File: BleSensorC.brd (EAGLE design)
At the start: 29 x 40.5 mm, 20 parts, among them IC1 PIC16LF18446-I_SS, IC2 SI7020-A20-GM, Q1 SI2333DDS-T1-GE3, T1 VEMT2523SLX01, U1 RN4871-I

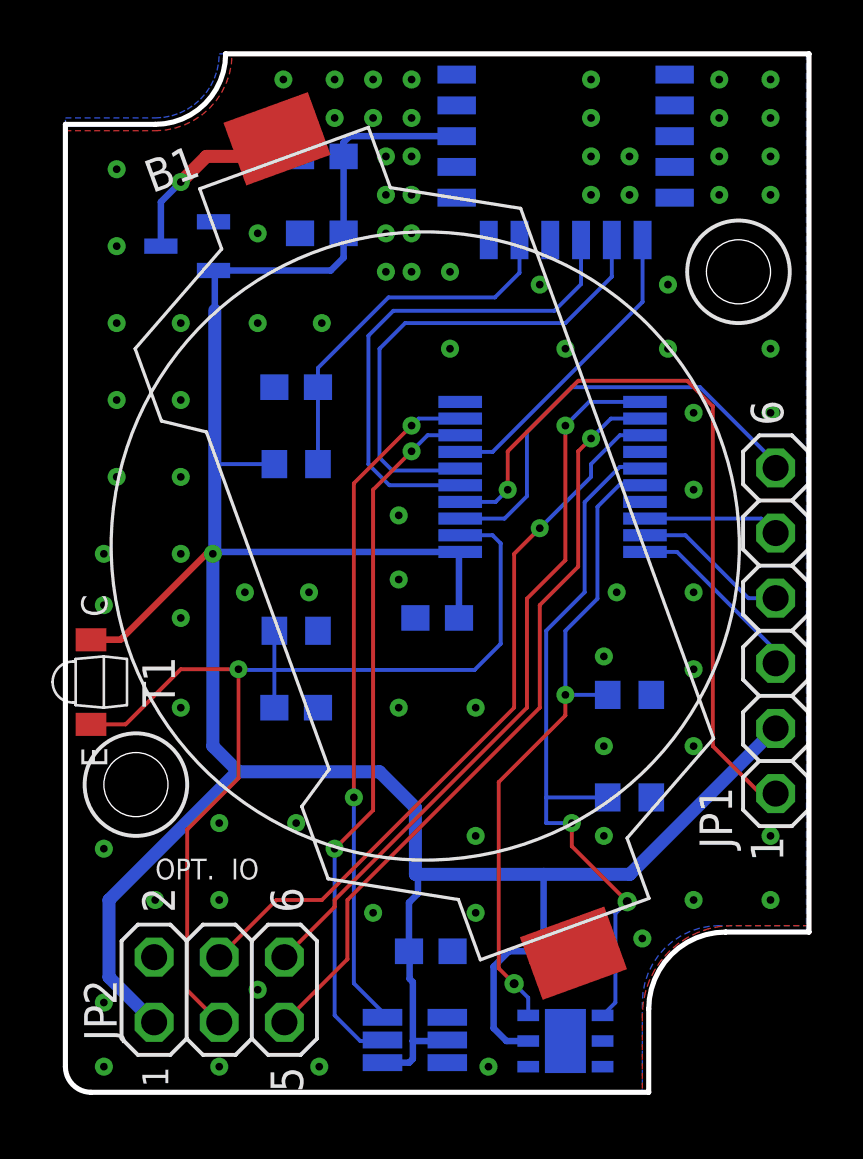
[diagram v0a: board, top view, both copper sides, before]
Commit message: U1 placing
U1 placing
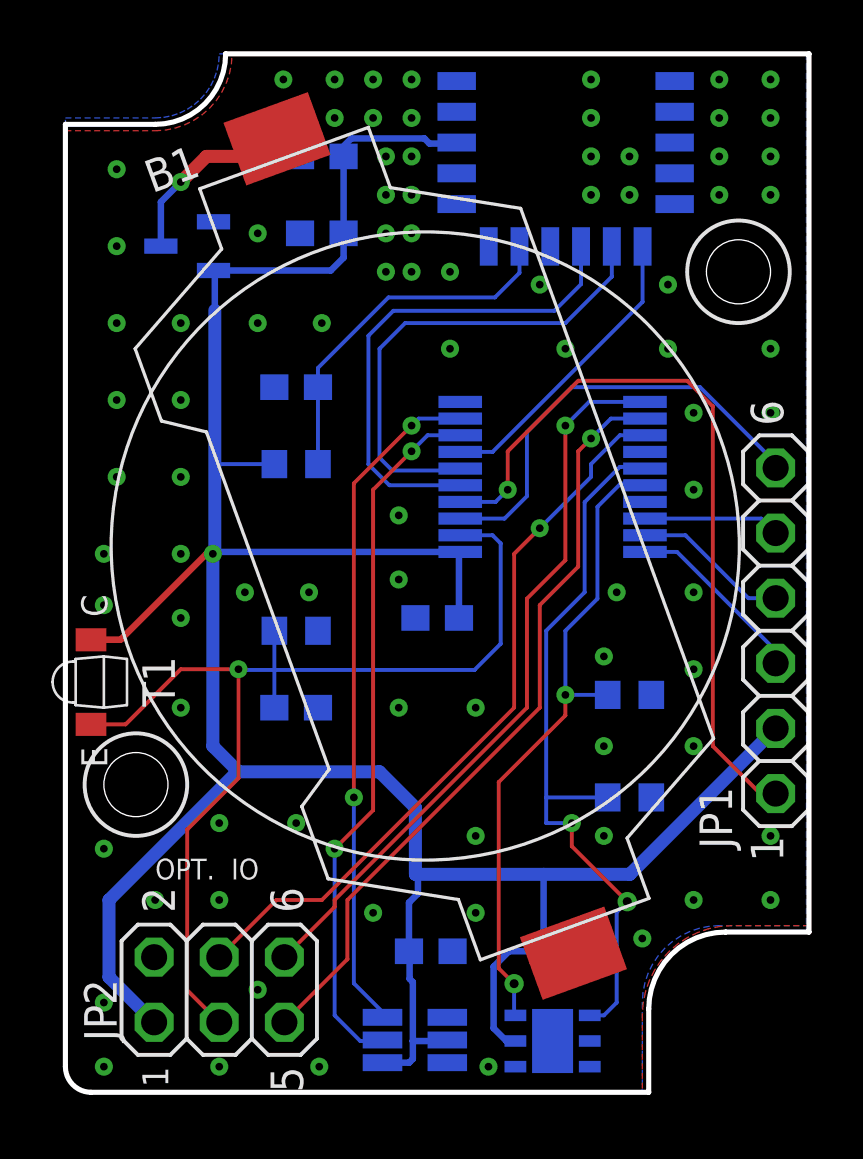
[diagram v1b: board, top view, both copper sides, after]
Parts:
- moved IC2 0.50 mm to (19.0, 2.00)
- moved U1 0.25 mm to (20.0, 37.2)
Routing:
- net SDA1: track 28.3 -> 28.8 mm
